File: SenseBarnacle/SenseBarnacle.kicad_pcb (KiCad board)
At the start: 4 copper layers, 82.6 x 35.5 mm, 108 parts, among them J1 USB_B_Mini, J2 Debug, J3 Power, J5 I2C_OLED_Display, J6 Conn_02x35_JumperluxCardEdge, J7 Conn_02x35_JumperluxCardEdge, SW1 USB BOOT, U1 LM324, U13 CH446X, U14 CH446X, U15 CH446X, U2 LM324, U3 NCP1117-3.3_SOT223, U6 AK4619VN, U8 W25Q128JVS, U9 RP2040, Y1 ABLS-12.000MHZ-B4-T

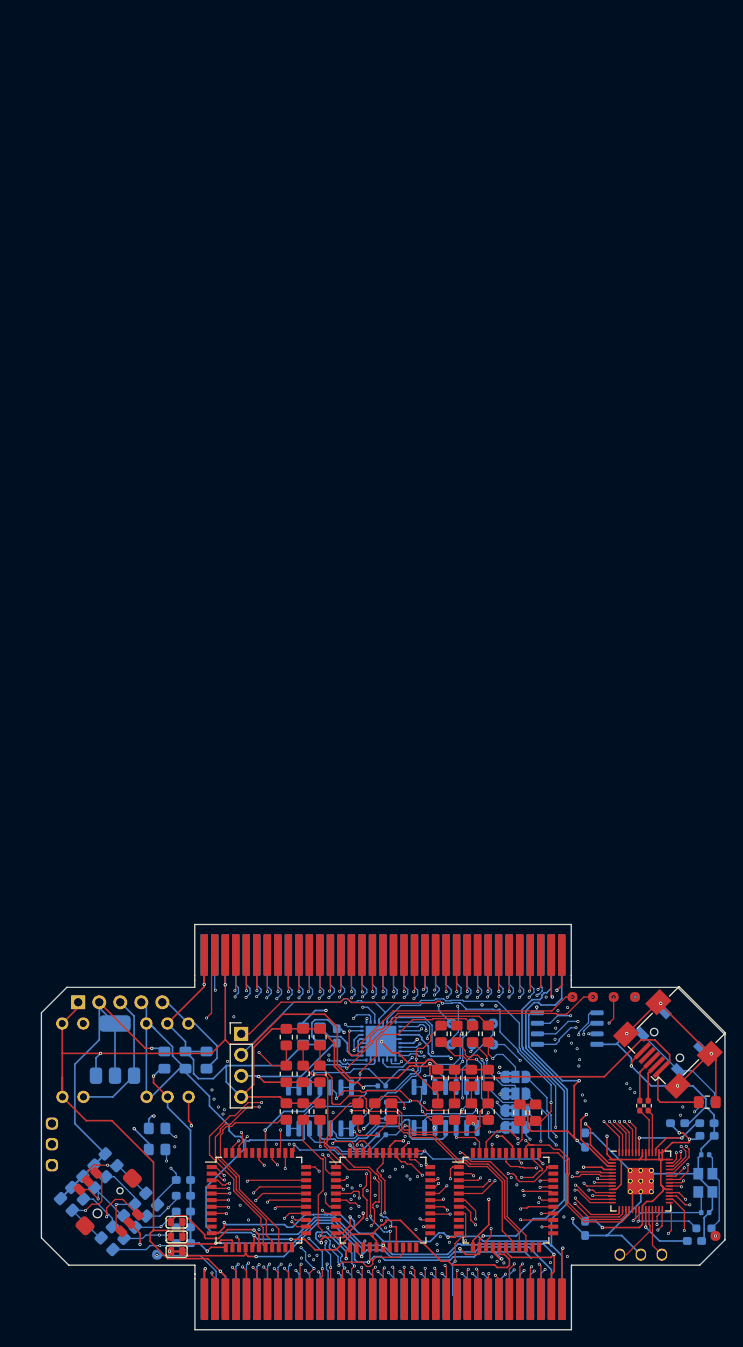
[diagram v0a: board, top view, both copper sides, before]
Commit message: Update SenseBarnacle.kicad_pcb
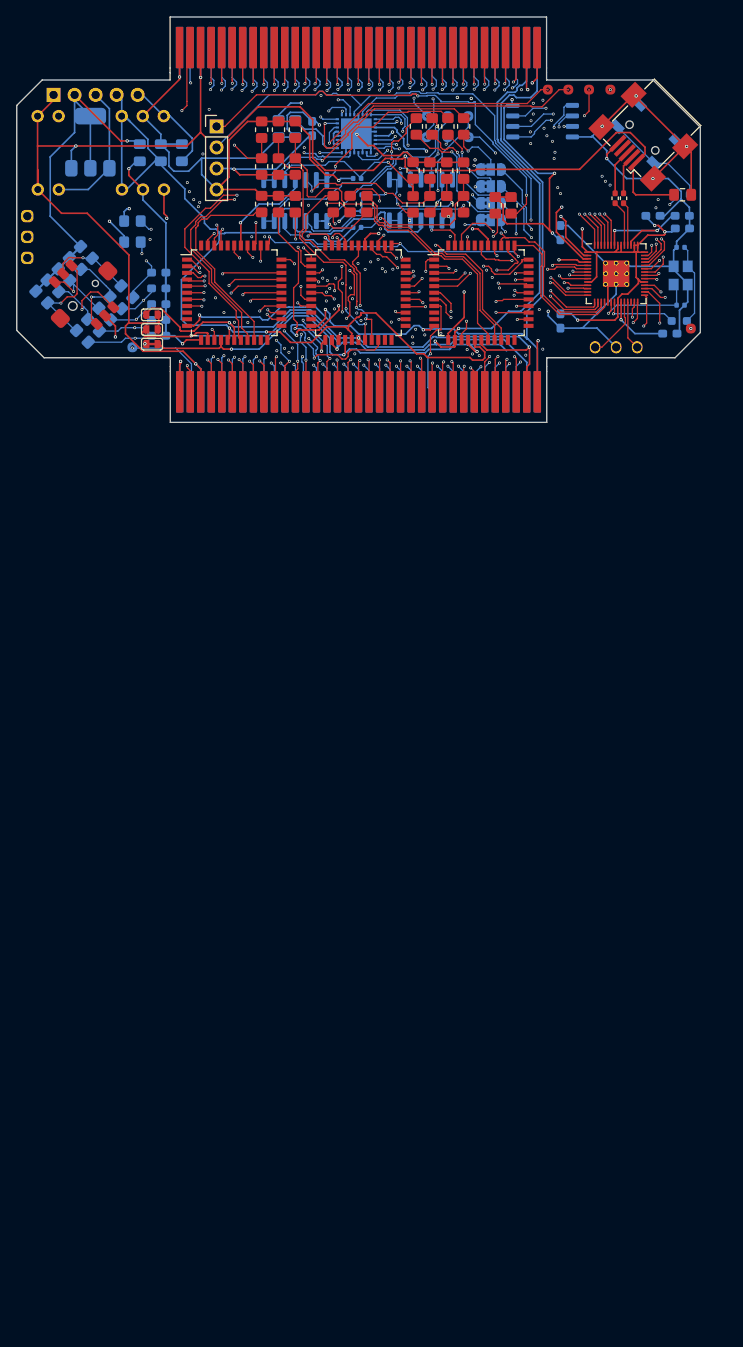
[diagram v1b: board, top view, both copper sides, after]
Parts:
- moved C6 109.6 mm to (117.2, 56.2)
- moved R13 109.6 mm to (86.9, 39.9)
- moved R15 109.6 mm to (89.0, 39.9)
- moved R17 109.6 mm to (91.0, 39.9)
- moved R5 109.6 mm to (40.0, 55.2)
- moved C1 109.6 mm to (117.4, 42.8)
- moved C12 109.6 mm to (102.7, 47.4)
- moved C14 109.6 mm to (78.1, 40.8)
- moved C15 109.6 mm to (79.2, 42.8)
- moved C18 109.6 mm to (54.2, 59.8)
- moved C23 109.6 mm to (54.2, 57.9)
- moved J3 109.6 mm to (41.5, 30.8)
- moved J5 109.6 mm to (61.2, 34.6)
- moved J7 109.6 mm to (78.3, 63.9)
- moved JP2 109.6 mm to (94.3, 45.9)
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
